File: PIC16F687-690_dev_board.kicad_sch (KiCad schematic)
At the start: 6 parts, among them J1 Conn_01x06_Pin, U1 PIC16F690-IP

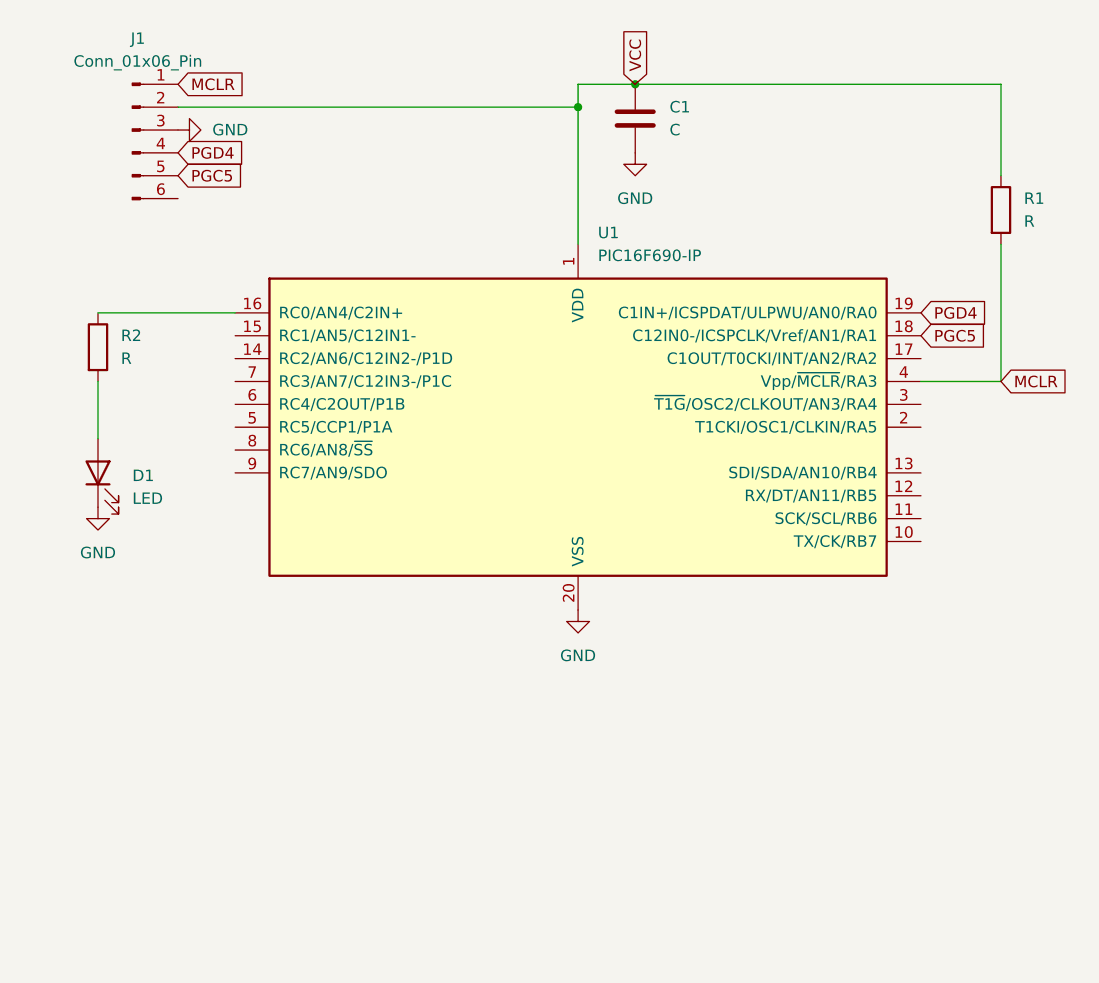
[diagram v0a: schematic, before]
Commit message: finalized layout organization
finalized layout organization
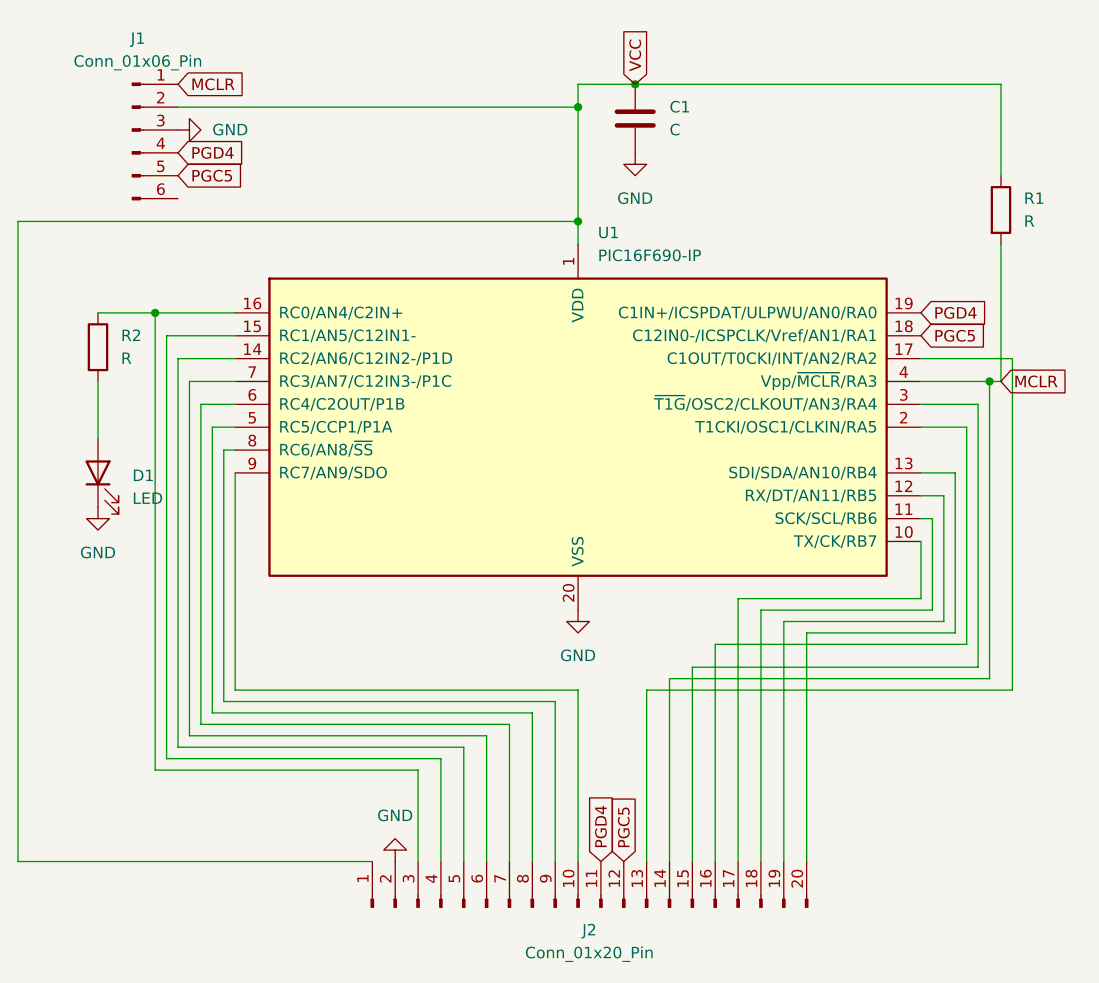
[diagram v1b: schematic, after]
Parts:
- added J2: Conn_01x20_Pin, Connector_PinHeader_2.54mm:PinHeader_1x20_P2.54mm_Vertical, symbol Connector:Conn_01x20_Pin
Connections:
- net GND: now also J2.2 (Pin_2)
- net MCLR: now also J2.14 (Pin_14)
- net PGC5: now also J2.12 (Pin_12)
- net PGD4: now also J2.11 (Pin_11)
- net VCC: now also J2.1 (Pin_1)
- net at U1.10 (TX/CK/RB7): now also J2.17 (Pin_17)
- net at U1.11 (SCK/SCL/RB6): now also J2.18 (Pin_18)
- net at U1.12 (RX/DT/AN11/RB5): now also J2.19 (Pin_19)
- net at U1.13 (SDI/SDA/AN10/RB4): now also J2.20 (Pin_20)
- net at U1.14 (RC2/AN6/C12IN2-/P1D): now also J2.5 (Pin_5)
- net at U1.15 (RC1/AN5/C12IN1-): now also J2.4 (Pin_4)
- net at R2.1, U1.16 (RC0/AN4/C2IN+): now also J2.3 (Pin_3)
- net at U1.17 (C1OUT/T0CKI/INT/AN2/RA2): now also J2.13 (Pin_13)
- net at U1.2 (T1CKI/OSC1/CLKIN/RA5): now also J2.16 (Pin_16)
- net at U1.3 (~{T1G}/OSC2/CLKOUT/AN3/RA4): now also J2.15 (Pin_15)
- net at U1.5 (RC5/CCP1/P1A): now also J2.8 (Pin_8)
- net at U1.6 (RC4/C2OUT/P1B): now also J2.7 (Pin_7)
- net at U1.7 (RC3/AN7/C12IN3-/P1C): now also J2.6 (Pin_6)
- net at U1.8 (RC6/AN8/~{SS}): now also J2.9 (Pin_9)
- net at U1.9 (RC7/AN9/SDO): now also J2.10 (Pin_10)
